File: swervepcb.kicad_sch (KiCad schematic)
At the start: 71 parts, among them J1 RJ45_LED, M1O1 PCB_Mounted_XT30, M1O2 PCB_Mounted_XT30, M2O1 PCB_Mounted_XT30, M2O2 PCB_Mounted_XT30, M3O1 PCB_Mounted_XT30, M3O2 PCB_Mounted_XT30, M4O1 PCB_Mounted_XT30, M4O2 PCB_Mounted_XT30, U0 BAT, U1 L298P, U2 L298P, U3 L298P, U4 L298P, U5 L7805, U6 NRF24L01_Breakout, U7 Teensy4.1

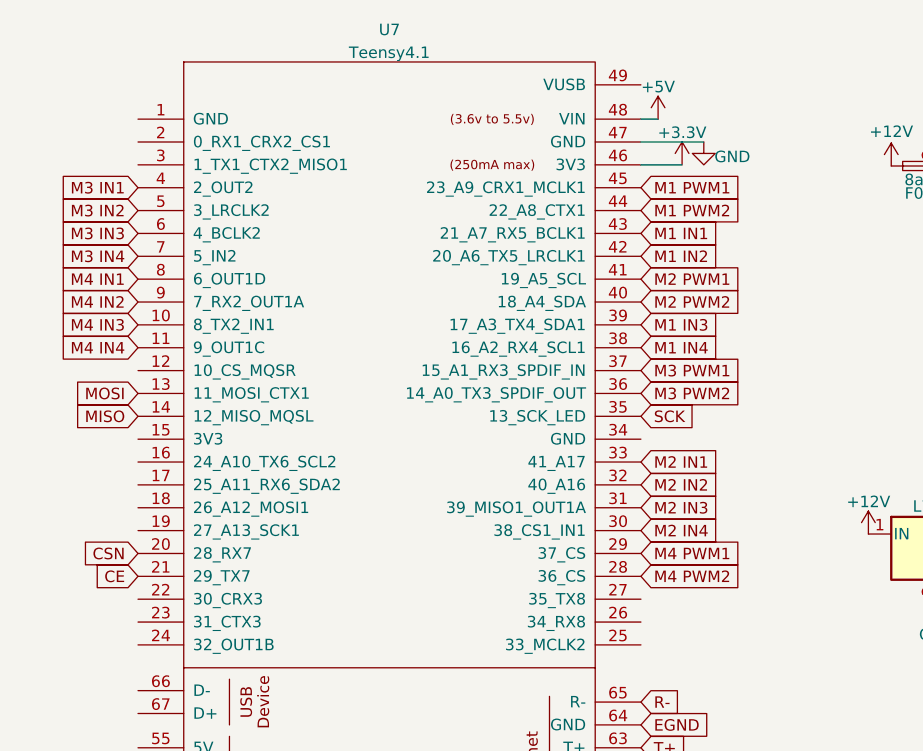
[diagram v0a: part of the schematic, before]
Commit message: progress
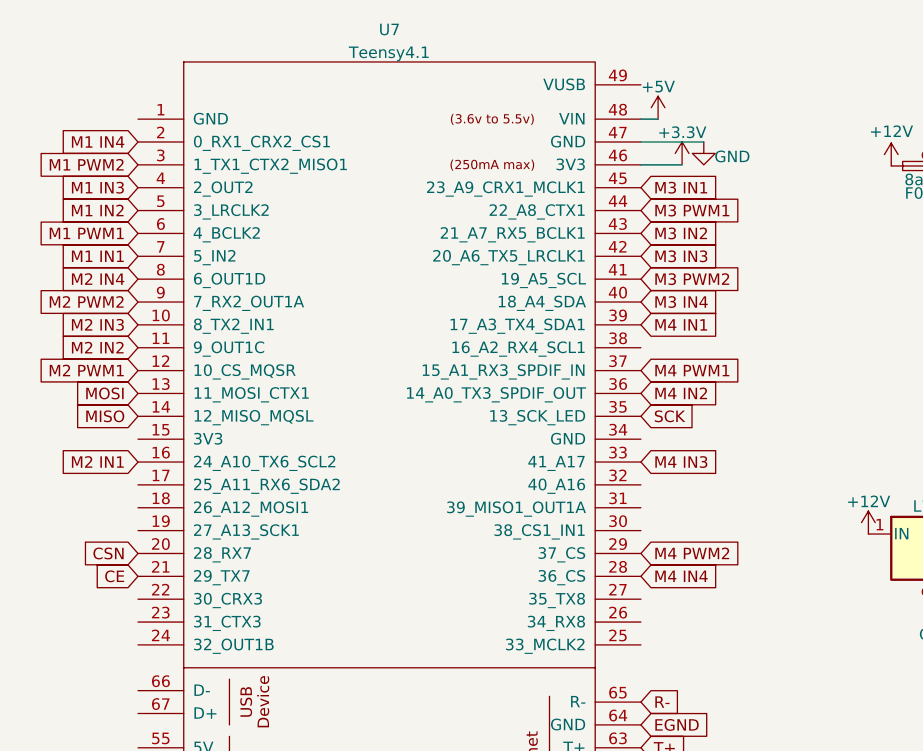
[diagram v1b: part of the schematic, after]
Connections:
- net M1 IN1: now also U7.7 (5_IN2); no longer U7.43 (21_A7_RX5_BCLK1)
- net M1 IN2: now also U7.5 (3_LRCLK2); no longer U7.42 (20_A6_TX5_LRCLK1)
- net M1 IN3: now also U7.4 (2_OUT2); no longer U7.39 (17_A3_TX4_SDA1)
- net M1 IN4: now also U7.2 (0_RX1_CRX2_CS1); no longer U7.38 (16_A2_RX4_SCL1)
- net M1 PWM1: now also U7.6 (4_BCLK2); no longer U7.45 (23_A9_CRX1_MCLK1)
- net M1 PWM2: now also U7.3 (1_TX1_CTX2_MISO1); no longer U7.44 (22_A8_CTX1)
- net M2 IN1: now also U7.16 (24_A10_TX6_SCL2); no longer U7.33 (41_A17)
- net M2 IN2: now also U7.11 (9_OUT1C); no longer U7.32 (40_A16)
- net M2 IN3: now also U7.10 (8_TX2_IN1); no longer U7.31 (39_MISO1_OUT1A)
- net M2 IN4: now also U7.8 (6_OUT1D); no longer U7.30 (38_CS1_IN1)
- net M2 PWM1: now also U7.12 (10_CS_MQSR); no longer U7.41 (19_A5_SCL)
- net M2 PWM2: now also U7.9 (7_RX2_OUT1A); no longer U7.40 (18_A4_SDA)
- net M3 IN1: now also U7.45 (23_A9_CRX1_MCLK1); no longer U7.4 (2_OUT2)
- net M3 IN2: now also U7.43 (21_A7_RX5_BCLK1); no longer U7.5 (3_LRCLK2)
- net M3 IN3: now also U7.42 (20_A6_TX5_LRCLK1); no longer U7.6 (4_BCLK2)
- net M3 IN4: now also U7.40 (18_A4_SDA); no longer U7.7 (5_IN2)
- net M3 PWM1: now also U7.44 (22_A8_CTX1); no longer U7.37 (15_A1_RX3_SPDIF_IN)
- net M3 PWM2: now also U7.41 (19_A5_SCL); no longer U7.36 (14_A0_TX3_SPDIF_OUT)
- net M4 IN1: now also U7.39 (17_A3_TX4_SDA1); no longer U7.8 (6_OUT1D)
- net M4 IN2: now also U7.36 (14_A0_TX3_SPDIF_OUT); no longer U7.9 (7_RX2_OUT1A)
- net M4 IN3: now also U7.33 (41_A17); no longer U7.10 (8_TX2_IN1)
- net M4 IN4: now also U7.28 (36_CS); no longer U7.11 (9_OUT1C)
- net M4 PWM1: now also U7.37 (15_A1_RX3_SPDIF_IN); no longer U7.29 (37_CS)
- net M4 PWM2: now also U7.29 (37_CS); no longer U7.28 (36_CS)
